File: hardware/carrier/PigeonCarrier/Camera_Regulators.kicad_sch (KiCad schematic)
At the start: 19 parts, among them U4 TPS62933FDRLR

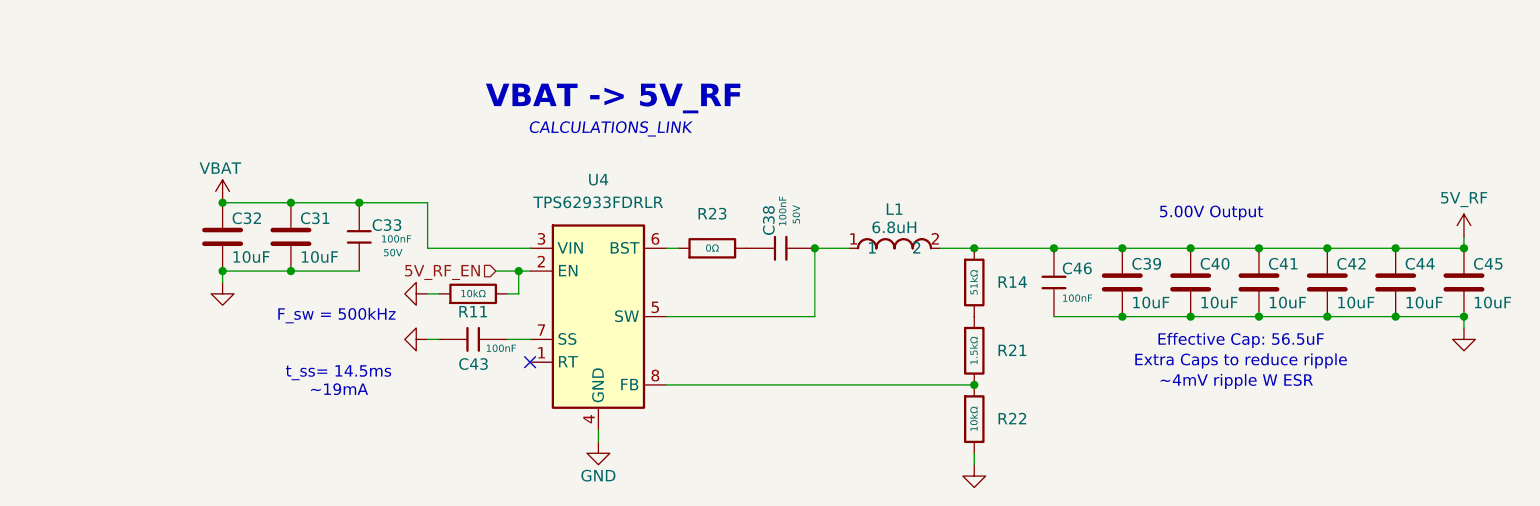
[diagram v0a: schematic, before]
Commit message: carrier progress
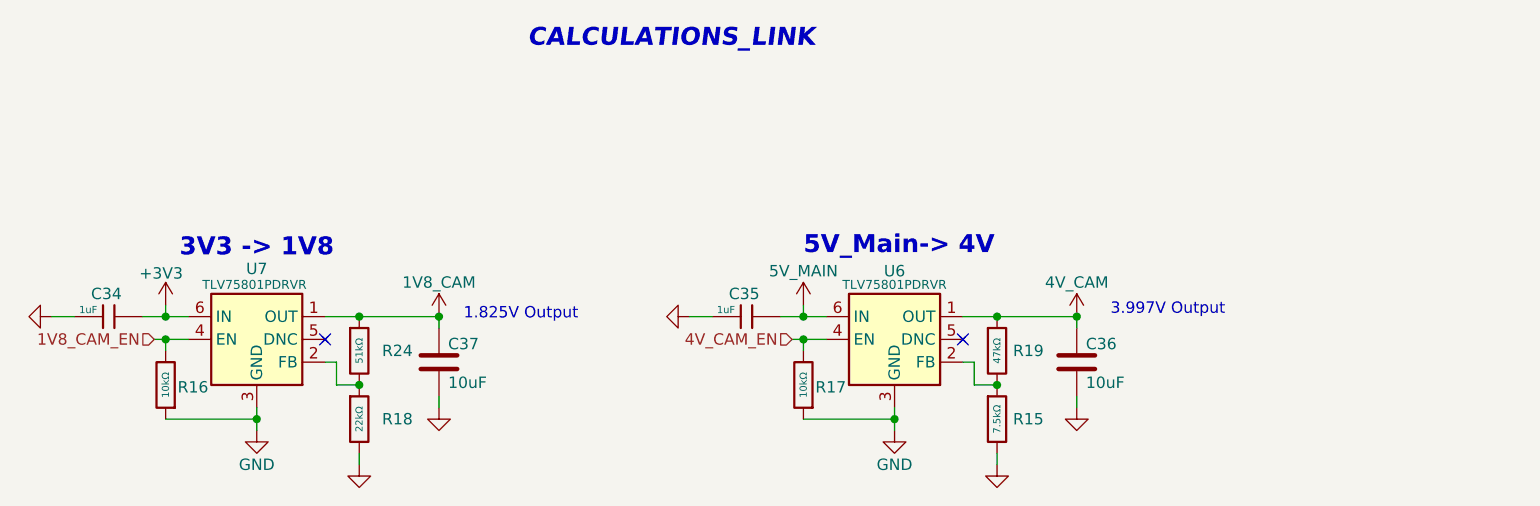
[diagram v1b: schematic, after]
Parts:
- removed C31, C32, C39, C40, C41, C42, C44, C45: 10uF, Capacitor_SMD:C_1210_3225Metric, symbol Device:C
- removed C33, C38, C43, C46: 100nF, PCM_JLCPCB:C_0402, symbol PCM_JLCPCB-Capacitors:0402,100nF,(2)
- removed L1: 6.8uH, JLCImport_Auto:CYA1040-6_8UH, symbol JLCImport_Auto:CYA1040-6_8UH
- removed R11, R22: 10kΩ, PCM_JLCPCB:R_0402, symbol PCM_JLCPCB-Resistors:0402,10kΩ
- removed R14: 51kΩ, PCM_JLCPCB:R_0402, symbol PCM_JLCPCB-Resistors:0402,51kΩ
- removed R21: 1.5kΩ, PCM_JLCPCB:R_0402, symbol PCM_JLCPCB-Resistors:0402,1.5kΩ
- removed R23: 0Ω, PCM_JLCPCB:R_0402, symbol PCM_JLCPCB-Resistors:0402,0Ω
- removed U4: TPS62933FDRLR, PigeonVision:SOT-583-8, symbol PigeonVision:TPS62933FDRLR
- added C34, C35: 1uF, PCM_JLCPCB:C_0603, symbol PCM_JLCPCB-Capacitors:0603,1uF
- added C36, C37: 10uF, Capacitor_SMD:C_1210_3225Metric, symbol Device:C
- added R15: 7.5kΩ, PCM_JLCPCB:R_0402, symbol PCM_JLCPCB-Resistors:0402,7.5kΩ
- added R16, R17: 10kΩ, PCM_JLCPCB:R_0402, symbol PCM_JLCPCB-Resistors:0402,10kΩ
- added R18: 22kΩ, PCM_JLCPCB:R_0402, symbol PCM_JLCPCB-Resistors:0402,22kΩ
- added R19: 47kΩ, PCM_JLCPCB:R_0402, symbol PCM_JLCPCB-Resistors:0402,47kΩ
- added R24: 51kΩ, PCM_JLCPCB:R_0402, symbol PCM_JLCPCB-Resistors:0402,51kΩ
- added U6, U7: TLV75801PDRVR, PigeonVision:TI_DRV0006A_WSON-6-1EP_2x2mm_P0.65mm, symbol PigeonVision:TLV75801PDRVR
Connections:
- net GND: now also C34.1, C35.1, C36.2, C37.2, R15.2, R16.1, R17.1, R18.2, U6.3 (GND), U6.7 (GND), U7.3 (GND), U7.7 (GND)
- new net: R15.1, R19.2, U6.2 (FB)
- new net: R18.1, R24.2, U7.2 (FB)
- new net +3V3: C34.2, U7.6 (IN)
- new net 1V8_CAM: C37.1, R24.1, U7.1 (OUT)
- new net 1V8_CAM_EN: R16.2, U7.4 (EN)
- new net 4V_CAM: C36.1, R19.1, U6.1 (OUT)
- new net 4V_CAM_EN: R17.2, U6.4 (EN)
- new net 5V_MAIN: C35.2, U6.6 (IN)
- no-connect marks 1 -> 2
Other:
- note added: "1.825V Output"
- note added: "3.997V Output"
- note added: "3V3 -> 1V8"
- note added: "5V_Main-> 4V"
- note removed: "5.00V Output"
- note removed: "Effective Cap: 56.5uF"
- note removed: "Extra Caps to reduce ripple"
- note removed: "F_sw = 500kHz"
- note removed: "VBAT -> 5V_RF"
- note removed: "t_ss= 14.5ms ~19mA"
- note removed: "~4mV ripple W ESR"
